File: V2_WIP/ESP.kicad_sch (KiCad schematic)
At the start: 36 parts, among them J202 USB4145-03-0230-C, Q1 IRLML5203, Q2 S8050, Q3 S8050, SW2 PTS647SN70SMTR2N LFS, U1 ESP32-WROOM-32UE, U14 *CH340K, U201 RT9080-33GJ5

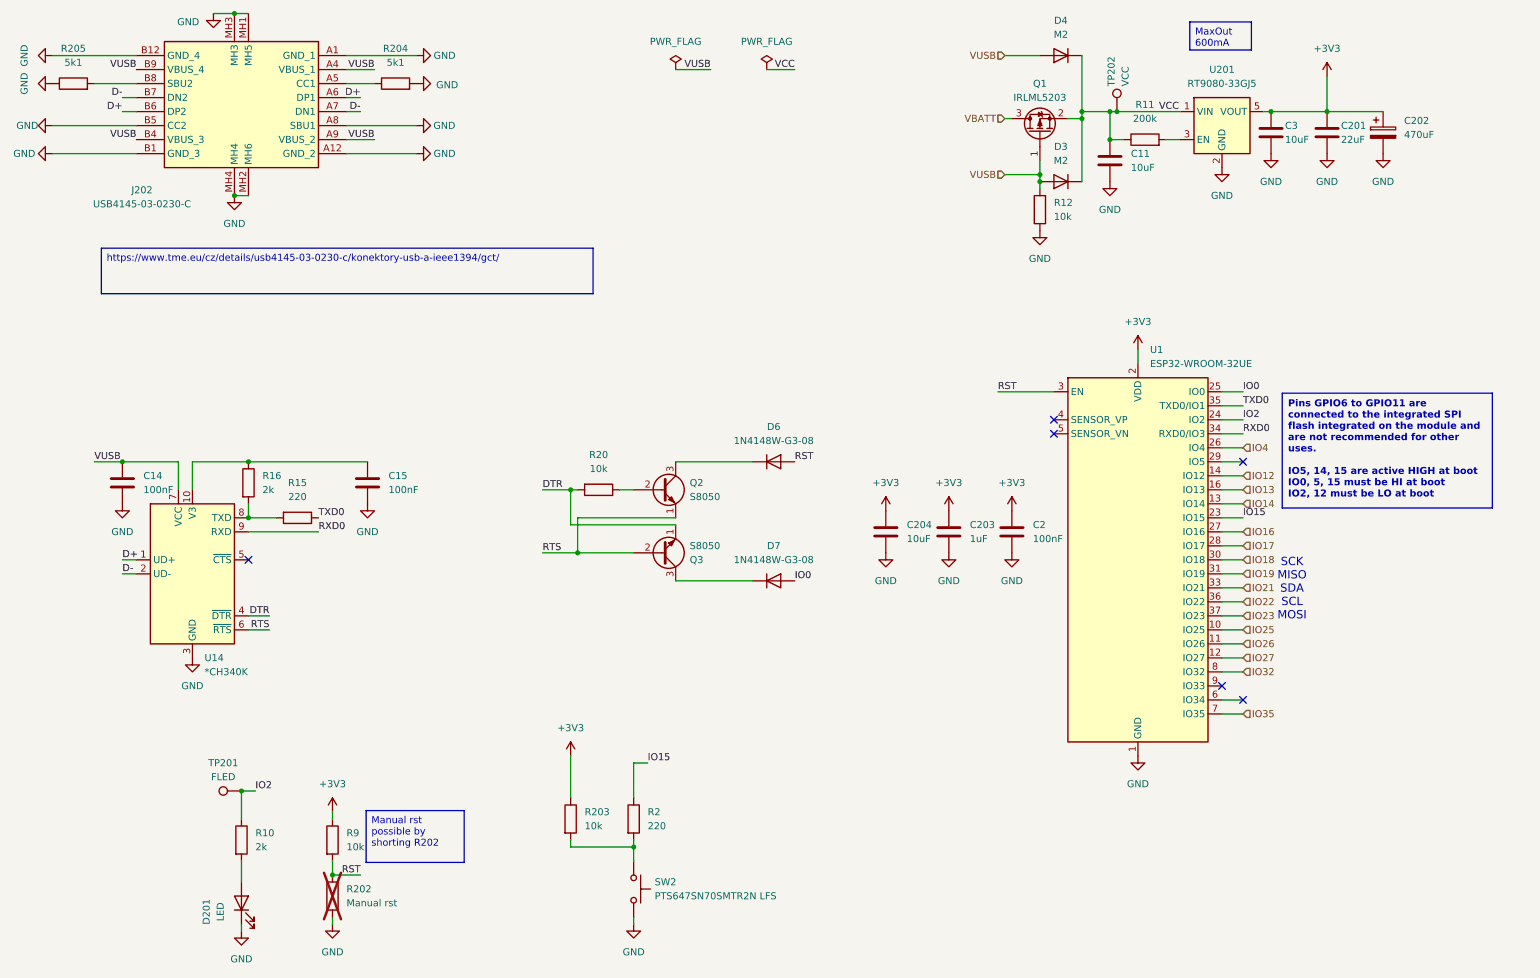
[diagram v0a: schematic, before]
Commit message: updated list of changes in README.md
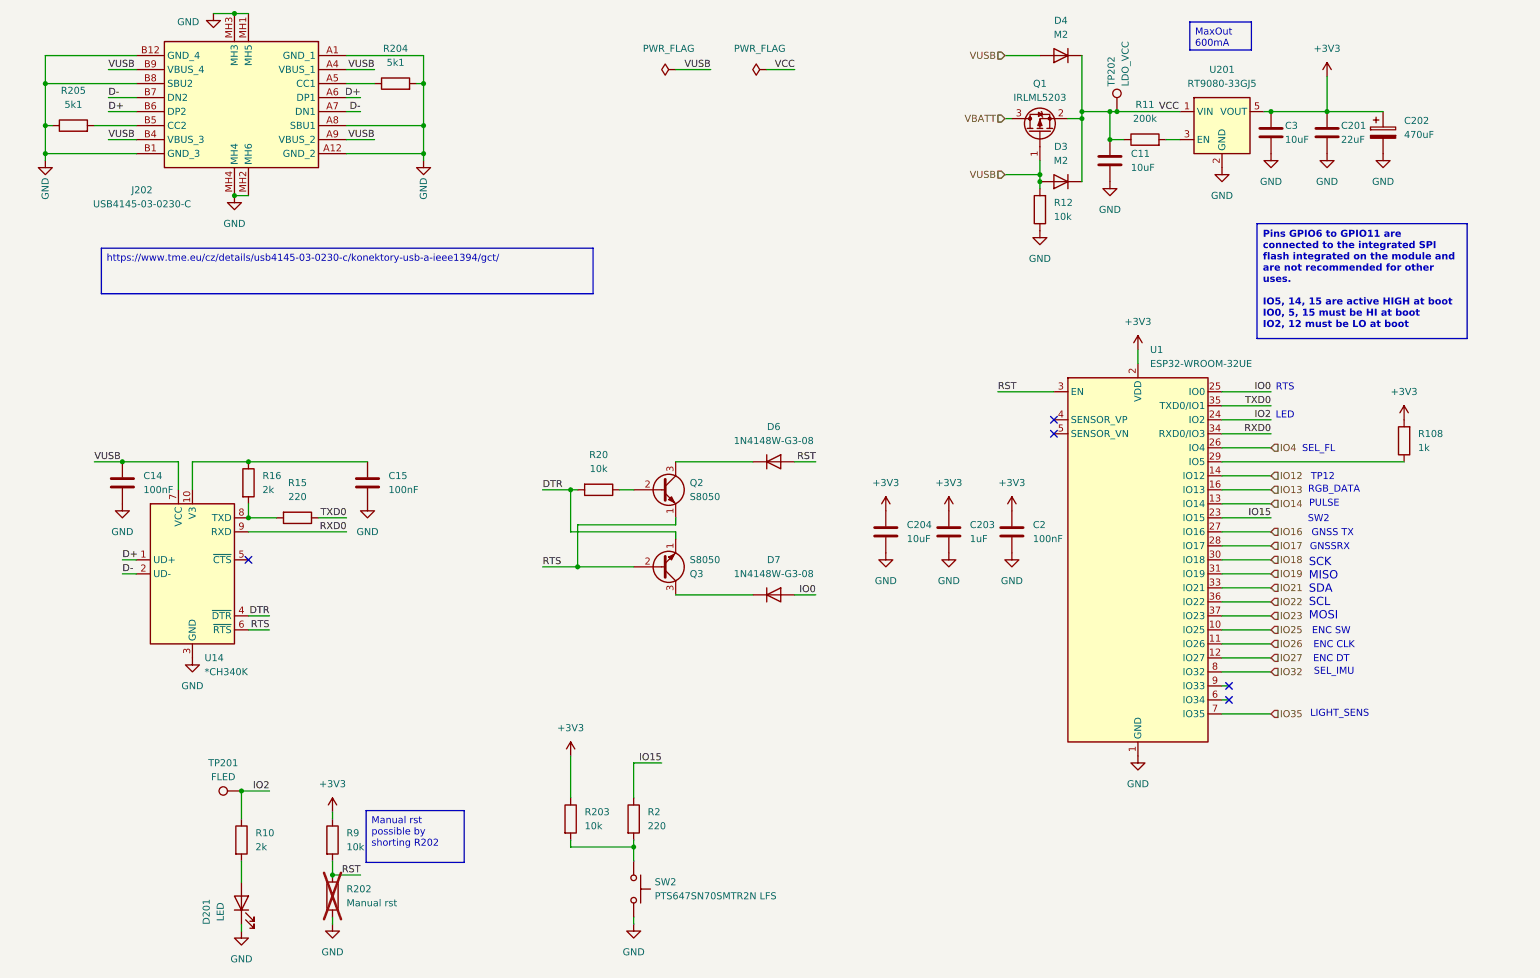
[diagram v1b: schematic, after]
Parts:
- added R108: 1k, Resistor_SMD:R_0603_1608Metric_Pad0.98x0.95mm_HandSolder, symbol Device:R
- TP201: footprint TestPoint:TestPoint_Pad_D1.5mm -> TestPoint:TestPoint_Pad_D1.0mm
- TP202: value VCC -> LDO_VCC; footprint TestPoint:TestPoint_Pad_D1.5mm -> TestPoint:TestPoint_Pad_D1.0mm
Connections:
- net +3V3: now also R108.2
- net GND: now also J202.B8 (SBU2); no longer J202.B5 (CC2)
- net at R205.2: now also J202.B5 (CC2); no longer J202.B8 (SBU2)
- net at U1.29 (IO5): now also R108.1
- no-connect marks 6 -> 5
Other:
- note added: "ENC CLK"
- note added: "ENC DT"
- note added: "ENC SW"
- note added: "GNSS TX"
- note added: "GNSSRX"
- note added: "LED"
- note added: "LIGHT_SENS"
- note added: "PULSE"
- note added: "RGB_DATA"
- note added: "RTS"
- note added: "SEL_FL"
- note added: "SEL_IMU"
- note added: "SW2"
- note added: "TP12"
- moved on the sheet: D7, Q3
